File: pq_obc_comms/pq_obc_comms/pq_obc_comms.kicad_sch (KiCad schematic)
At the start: 66 parts, among them J1 Conn_01x10, J2 Conn_01x10, J3 Conn_01x10, J4 Conn_01x10, J6 U.FL-R-SMT-1_10_, U1 STM32L476RGTx, U2 SX1262IMLTRT, U3 BD2232G-GTR, U4 BD2232G-GTR, U5 RFswitch, U7 BD2232G-GTR, X1 12MHz, X2 FA-128_32.0000MF20X-K5, X3 32.768KHz

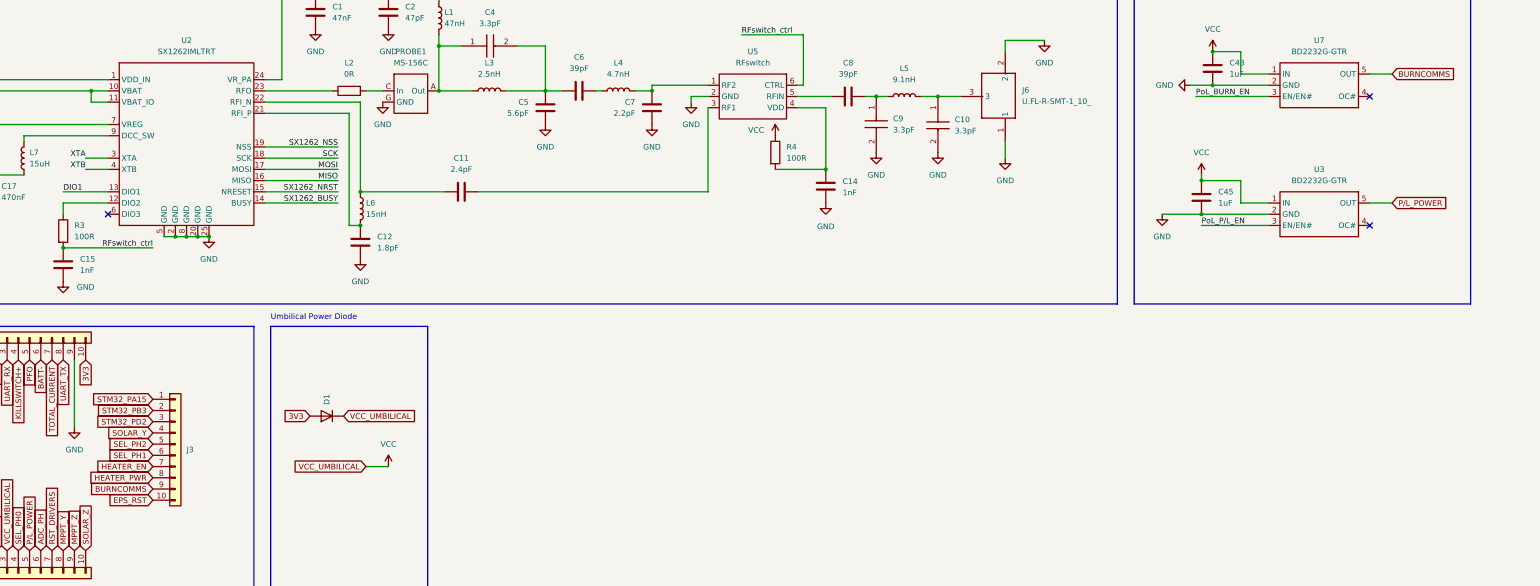
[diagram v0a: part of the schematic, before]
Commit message: Cleanup!
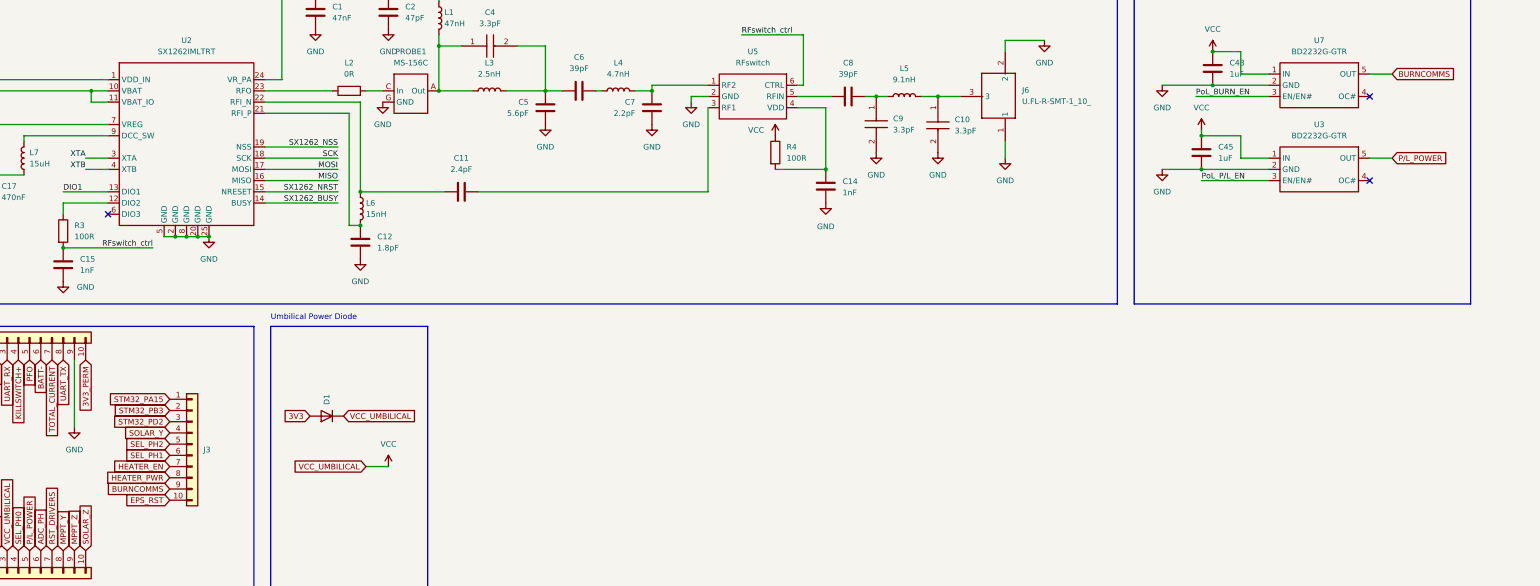
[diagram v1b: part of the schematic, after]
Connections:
- net 3V3: no longer J1.10 (Pin_10)
- new net 3V3_PERM: J1.10 (Pin_10)
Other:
- moved on the sheet: C45, J3, U3

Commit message: obc rework
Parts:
- removed C40, C41: 20pF, symbol COMMS-altium-import:3_20pF
- removed D2: VCC_TEST, symbol COMMS-altium-import:0_VCC_TEST
- removed J6: U.FL-R-SMT-1_10_, symbol COMMS-altium-import:1_U.FL-R-SMT-1_10_
- removed PROBE1: MS-156C, GGS_Connectors:CoaxialSwitch_Hirose_MS-156C3_Horizontal, symbol GGS_Connectors:MS-156C
- removed X1: 12MHz, GGS_Miscellaneous:ECX-32, symbol COMMS-altium-import:0_12MHz
- added C40: 20pF, Capacitor_SMD:C_0603_1608Metric, symbol COMMS-altium-import:3_10pF
- added C41: 20pF, Capacitor_SMD:C_0603_1608Metric, symbol COMMS-altium-import:3_100nF
- added D2: RBS1LAM40ATR, Diode_SMD:D_SOD-128, symbol Simulation_SPICE:DIODE
- added J6: U.FL-R-SMT-1_10, Connector_Coaxial:U.FL_Hirose_U.FL-R-SMT-1_Vertical, symbol Connector:Conn_Coaxial
- added TP1: CoaxialSwitch_Testpoint, symbol Connector:CoaxialSwitch_Testpoint
- added X1: ECS-120-18-33-JEM-TR3, GGS_Miscellaneous:ECX-32, symbol Device:Crystal_GND24
- C1, C11, C12, C2, C4, C5, C6, C7, C8: footprint (none) -> Capacitor_SMD:C_0402_1005Metric
- C10, C9: footprint (none) -> Capacitor_SMD:C_0402_1005Metric; symbol COMMS-altium-import:3_3.3pF -> Device:C
- C14, C15, C16, C17, C18, C27, C28, C42, C43, C44, C45: footprint (none) -> Capacitor_SMD:C_0603_1608Metric
- D1: value VCC -> RBS1LAM40ATR; footprint (none) -> Diode_SMD:D_SOD-128; BOM_JLCPCB PART CLASS Extended Part -> (none); BOM_MANUFACTURER ROHM Semicon -> (none); BOM_MANUFACTURER PART PDZVTR4.7B -> (none); BOM_SUPPLIER LCSC -> (none); BOM_SUPPLIER PART C253498 -> (none)
- L1, L2, L3, L4, L5, L6: footprint (none) -> Inductor_SMD:L_0402_1005Metric
- L7: footprint (none) -> Inductor_SMD:L_0805_2012Metric
- R3, R4, R6, R7, R8: footprint (none) -> Resistor_SMD:R_0603_1608Metric
- U2: footprint (none) -> Package_DFN_QFN:QFN-24-1EP_4x4mm_P0.5mm_EP2.6x2.6mm
- U3, U4, U7: footprint (none) -> Package_TO_SOT_SMD:SOT-23-5
- U5: value RFswitch -> BGS12PL6E6327XTSA1; footprint (none) -> GGS_RF:PG-TSLP-6-4; BOM_SUPPLIER PART C1854968 -> BGS12PL6E6327XTSA1
- X3: value 32.768KHz -> ABS09-32.768KHZ-7-T; footprint (none) -> GGS_Miscellaneous:ABS09; BOM_SUPPLIER LCSC -> (none); BOM_SUPPLIER PART C1985392 -> (none)
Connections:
- net ADC_PH: now also J4.5 (Pin_5); no longer J4.6 (Pin_6)
- net ADC_PL: now also J2.9 (Pin_9); no longer J2.2 (Pin_2)
- net CHRG: now also J4.10 (Pin_10); no longer J4.1 (Pin_1)
- net CHRGOFF: now also J2.4 (Pin_4); no longer J2.7 (Pin_7)
- net CLPROG: now also J2.3 (Pin_3); no longer J2.8 (Pin_8)
- net DAC_PL: now also J2.8 (Pin_8); no longer J2.3 (Pin_3)
- net EPS_RST: no longer J3.10 (Pin_10)
- net FAULT: now also J4.9 (Pin_9); no longer J4.2 (Pin_2)
- net GND: now also C40.2, C41.2, J6.2 (Ext), TP1.G, X1.2, X1.4
- net MPPT_X: no longer J2.9 (Pin_9)
- net MPPT_Y: no longer J4.8 (Pin_8)
- net MPPT_Z: no longer J4.9 (Pin_9)
- net NRST: now also J2.5 (Pin_5); no longer J2.6 (Pin_6)
- net OSC_IN: now also C40.1, X1.1
- net OSC_OUT: now also C41.1, X1.3
- net P/L_POWER: now also J4.6 (Pin_6); no longer J4.5 (Pin_5)
- net RST_DRIVERS: now also J4.4 (Pin_4); no longer J4.7 (Pin_7)
- net SEL_PH0: now also J4.7 (Pin_7); no longer J4.4 (Pin_4)
- net SOLAR_X: now also J2.1 (Pin_1); no longer J2.10 (Pin_10)
- net SOLAR_Z: now also J4.1 (Pin_1); no longer J4.10 (Pin_10)
- net STM32_PA2: now also J2.10 (Pin_10); no longer J2.1 (Pin_1)
- net STM32_PD2: now also J4.2 (Pin_2); no longer J3.3 (Pin_3)
- net SWCLK: now also J2.7 (Pin_7); no longer J2.4 (Pin_4)
- net SWDIO: now also J2.6 (Pin_6); no longer J2.5 (Pin_5)
- net VCC: now also D2.2 (K); no longer J4.3 (Pin_3)
- net at L2.2: now also TP1.C
- net at C10.1, L5.2: now also J6.1 (In)
- net at C4.1, L1.2, L3.1: now also TP1.A
- net P/L2BURN renamed ADCS_POWER
- net ADCS_POWER: now also J4.3 (Pin_3)
- new net BATT_NTC: J3.3 (Pin_3)
- new net VCC_UMBILICAL: D2.1 (A), J4.8 (Pin_8)
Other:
- note removed: "To be done in PL2 board"
- note removed: "Vcc Test"
- moved on the sheet: C1, C14, C2, C27, C28, C31, C32, C33, C34, C35, C36, C37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
